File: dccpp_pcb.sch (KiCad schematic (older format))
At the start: 60 parts, among them J1 USB_B_Micro, J10 OSTTC022162, J11 OSTTC022162, J12 OSTTC022162, J2 AVR-ISP-6, J3 OSTTC022162, J4 OSTTC022162, J5 OSTTC022162, J6 OSTTC022162, J7 OSTTC022162, J8 OSTTC022162, J9 OSTTC022162, U1 ATmega32U4-AU, U2 74HC04, U3 IFX007T, U4 IFX007T, U5 IFX007T, U6 IFX007T, Y1 16MHz

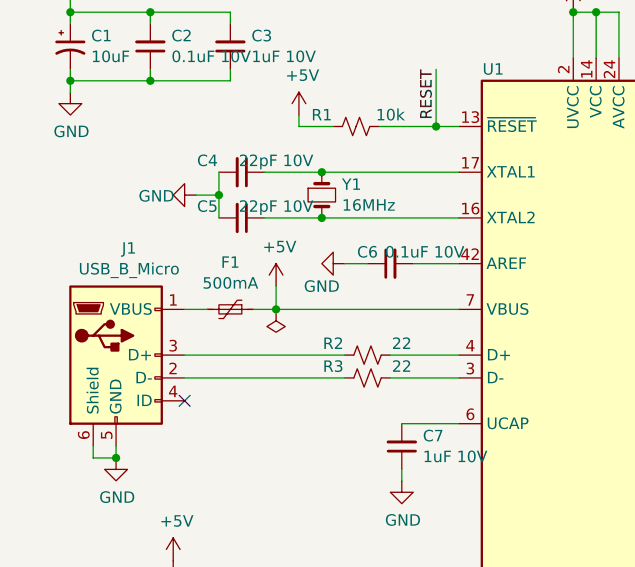
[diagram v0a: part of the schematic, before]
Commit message: Final part numbers
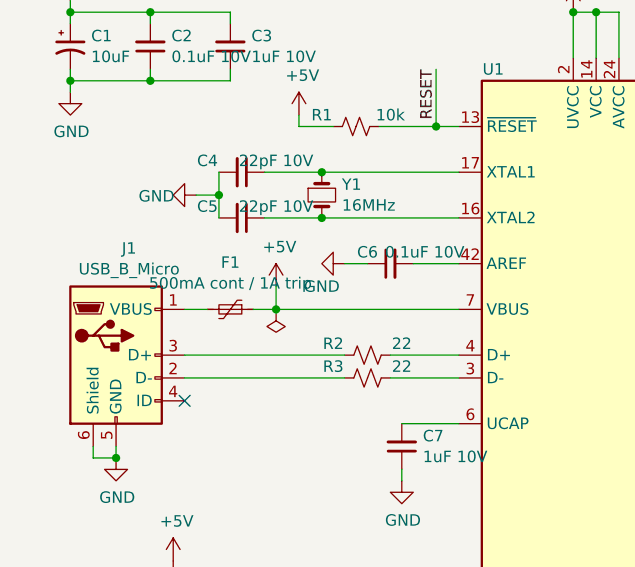
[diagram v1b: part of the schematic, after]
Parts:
- D1: Digi-Key_PN (none) -> 732-12018-1-ND; MPN (none) -> 150060YS55040
- D2: Digi-Key_PN (none) -> 732-12017-1-ND; MPN (none) -> 150060VS55040
- F1: value 500mA -> 500mA cont / 1A trip; footprint (none) -> Fuse:Fuse_1206_3216Metric_Pad1.42x1.75mm_HandSolder; Digi-Key_PN (none) -> 507-1802-1-ND; MPN (none) -> 0ZCJ0050FF2G
- J2: Digi-Key_PN (none) -> 609-5122-ND; MPN (none) -> 75869-331LF
- R1, R10, R11, R12, R13, R14, R15, R16, R6, R9: Digi-Key_PN (none) -> RNCP0603FTD10K0CT-ND; MPN (none) -> RNCP0603FTD10K0
- R17, R18, R19, R20: Digi-Key_PN (none) -> 311-510HRCT-ND; MPN (none) -> RC0603FR-07510RL
- R2, R3: Digi-Key_PN (none) -> 311-22.0HRCT-ND; MPN (none) -> RC0603FR-0722RL
- R4, R5: Digi-Key_PN (none) -> 311-330HRCT-ND; MPN (none) -> RC0603FR-07330RL
- R7, R8: Digi-Key_PN (none) -> 311-470HRCT-ND; MPN (none) -> RC0603FR-07470RL
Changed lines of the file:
@@
 F 2 "Resistor_SMD:R_0603_1608Metric_Pad1.05x0.95mm_HandSolder" H 2000 2400 50  0001 C CNN
 F 3 "~" H 2000 2400 50  0001 C CNN
+F 4 "311-22.0HRCT-ND" H 2000 2400 50  0001 C CNN "Digi-Key_PN"
+F 5 "RC0603FR-0722RL" H 2000 2400 50  0001 C CNN "MPN"
 	1    2000 2400
 	0    1    1    0
@@
 P 1400 2100
 F 0 "F1" V 1195 2100 50  0000 C CNN
-F 1 "500mA" V 1286 2100 50  0000 C CNN
-F 2 "" H 1450 1900 50  0001 L CNN
+F 1 "500mA cont / 1A trip" V 1286 2100 50  0000 C CNN
+F 2 "Fuse:Fuse_1206_3216Metric_Pad1.42x1.75mm_HandSolder" H 1450 1900 50  0001 L CNN
 F 3 "~" H 1400 2100 50  0001 C CNN
+F 4 "507-1802-1-ND" H 1400 2100 50  0001 C CNN "Digi-Key_PN"
+F 5 "0ZCJ0050FF2G" H 1400 2100 50  0001 C CNN "MPN"
 	1    1400 2100
 	0    1    1    0
@@
 F 2 "Resistor_SMD:R_0603_1608Metric_Pad1.05x0.95mm_HandSolder" H 1950 1300 50  0001 C CNN
 F 3 "~" H 1950 1300 50  0001 C CNN
+F 4 "RNCP0603FTD10K0CT-ND" H 1950 1300 50  0001 C CNN "Digi-Key_PN"
+F 5 "RNCP0603FTD10K0" H 1950 1300 50  0001 C CNN "MPN"
 	1    1950 1300
 	0    1    1    0
@@
 F 2 "Resistor_SMD:R_0603_1608Metric_Pad1.05x0.95mm_HandSolder" H 2000 2300 50  0001 C CNN
 F 3 "~" H 2000 2300 50  0001 C CNN
+F 4 "311-22.0HRCT-ND" H 2000 2300 50  0001 C CNN "Digi-Key_PN"
+F 5 "RC0603FR-0722RL" H 2000 2300 50  0001 C CNN "MPN"
 	1    2000 2300
 	0    1    1    0
@@
 F 2 "Connector_IDC:IDC-Header_2x03_P2.54mm_Vertical" V 1000 3750 50  0001 C CNN
 F 3 " ~" H -25 3150 50  0001 C CNN
+F 4 "609-5122-ND" H 1250 3700 50  0001 C CNN "Digi-Key_PN"
+F 5 "75869-331LF" H 1250 3700 50  0001 C CNN "MPN"
 	1    1250 3700
 	1    0    0    -1
@@
 F 2 "Resistor_SMD:R_0603_1608Metric_Pad1.05x0.95mm_HandSolder" H 9150 2100 50  0001 C CNN
 F 3 "~" H 9150 2100 50  0001 C CNN
+F 4 "311-510HRCT-ND" H 9150 2100 50  0001 C CNN "Digi-Key_PN"
+F 5 "RC0603FR-07510RL" H 9150 2100 50  0001 C CNN "MPN"
 	1    9150 2100
 	1    0    0    -1
@@
 F 2 "Resistor_SMD:R_0603_1608Metric_Pad1.05x0.95mm_HandSolder" H 9100 3000 50  0001 C CNN
 F 3 "~" H 9100 3000 50  0001 C CNN
+F 4 "311-510HRCT-ND" H 9100 3000 50  0001 C CNN "Digi-Key_PN"
+F 5 "RC0603FR-07510RL" H 9100 3000 50  0001 C CNN "MPN"
 	1    9100 3000
 	1    0    0    -1
@@
 F 2 "Resistor_SMD:R_0603_1608Metric_Pad1.05x0.95mm_HandSolder" H 9100 4100 50  0001 C CNN
 F 3 "~" H 9100 4100 50  0001 C CNN
+F 4 "311-510HRCT-ND" H 9100 4100 50  0001 C CNN "Digi-Key_PN"
+F 5 "RC0603FR-07510RL" H 9100 4100 50  0001 C CNN "MPN"
 	1    9100 4100
 	1    0    0    -1
@@
 F 2 "Resistor_SMD:R_0603_1608Metric_Pad1.05x0.95mm_HandSolder" H 9100 5000 50  0001 C CNN
 F 3 "~" H 9100 5000 50  0001 C CNN
+F 4 "311-510HRCT-ND" H 9100 5000 50  0001 C CNN "Digi-Key_PN"
+F 5 "RC0603FR-07510RL" H 9100 5000 50  0001 C CNN "MPN"
 	1    9100 5000
 	1    0    0    -1
@@
 F 2 "Resistor_SMD:R_0603_1608Metric_Pad1.05x0.95mm_HandSolder" H 9050 1700 50  0001 C CNN
 F 3 "~" H 9050 1700 50  0001 C CNN
+F 4 "RNCP0603FTD10K0CT-ND" H 9050 1700 50  0001 C CNN "Digi-Key_PN"
+F 5 "RNCP0603FTD10K0" H 9050 1700 50  0001 C CNN "MPN"
 	1    9050 1700
 	0    1    1    0
@@
 F 2 "Resistor_SMD:R_0603_1608Metric_Pad1.05x0.95mm_HandSolder" H 9050 1800 50  0001 C CNN
 F 3 "~" H 9050 1800 50  0001 C CNN
+F 4 "RNCP0603FTD10K0CT-ND" H 9050 1800 50  0001 C CNN "Digi-Key_PN"
+F 5 "RNCP0603FTD10K0" H 9050 1800 50  0001 C CNN "MPN"
 	1    9050 1800
 	0    1    1    0
@@
 F 2 "Resistor_SMD:R_0603_1608Metric_Pad1.05x0.95mm_HandSolder" H 9050 2600 50  0001 C CNN
 F 3 "~" H 9050 2600 50  0001 C CNN
+F 4 "RNCP0603FTD10K0CT-ND" H 9050 2600 50  0001 C CNN "Digi-Key_PN"
+F 5 "RNCP0603FTD10K0" H 9050 2600 50  0001 C CNN "MPN"
 	1    9050 2600
 	0    1    1    0
@@
 F 2 "Resistor_SMD:R_0603_1608Metric_Pad1.05x0.95mm_HandSolder" H 9050 2700 50  0001 C CNN
 F 3 "~" H 9050 2700 50  0001 C CNN
+F 4 "RNCP0603FTD10K0CT-ND" H 9050 2700 50  0001 C CNN "Digi-Key_PN"
+F 5 "RNCP0603FTD10K0" H 9050 2700 50  0001 C CNN "MPN"
 	1    9050 2700
 	0    1    1    0
@@
 F 2 "Resistor_SMD:R_0603_1608Metric_Pad1.05x0.95mm_HandSolder" H 9050 3700 50  0001 C CNN
 F 3 "~" H 9050 3700 50  0001 C CNN
+F 4 "RNCP0603FTD10K0CT-ND" H 9050 3700 50  0001 C CNN "Digi-Key_PN"
+F 5 "RNCP0603FTD10K0" H 9050 3700 50  0001 C CNN "MPN"
 	1    9050 3700
 	0    1    1    0
@@
 F 2 "Resistor_SMD:R_0603_1608Metric_Pad1.05x0.95mm_HandSolder" H 9050 3800 50  0001 C CNN
 F 3 "~" H 9050 3800 50  0001 C CNN
+F 4 "RNCP0603FTD10K0CT-ND" H 9050 3800 50  0001 C CNN "Digi-Key_PN"
+F 5 "RNCP0603FTD10K0" H 9050 3800 50  0001 C CNN "MPN"
 	1    9050 3800
 	0    1    1    0
@@
 F 2 "Resistor_SMD:R_0603_1608Metric_Pad1.05x0.95mm_HandSolder" H 9050 4600 50  0001 C CNN
 F 3 "~" H 9050 4600 50  0001 C CNN
+F 4 "RNCP0603FTD10K0CT-ND" H 9050 4600 50  0001 C CNN "Digi-Key_PN"
+F 5 "RNCP0603FTD10K0" H 9050 4600 50  0001 C CNN "MPN"
 	1    9050 4600
 	0    1    1    0
@@
 F 2 "Resistor_SMD:R_0603_1608Metric_Pad1.05x0.95mm_HandSolder" H 9050 4700 50  0001 C CNN
 F 3 "~" H 9050 4700 50  0001 C CNN
+F 4 "RNCP0603FTD10K0CT-ND" H 9050 4700 50  0001 C CNN "Digi-Key_PN"
+F 5 "RNCP0603FTD10K0" H 9050 4700 50  0001 C CNN "MPN"
 	1    9050 4700
 	0    1    1    0
@@
 F 2 "LED_SMD:LED_0603_1608Metric_Pad1.05x0.95mm_HandSolder" H 4300 3000 50  0001 C CNN
 F 3 "~" H 4300 3000 50  0001 C CNN
+F 4 "732-12017-1-ND" H 4300 3000 50  0001 C CNN "Digi-Key_PN"
+F 5 "150060VS55040" H 4300 3000 50  0001 C CNN "MPN"
 	1    4300 3000
 	1    0    0    -1
@@
 F 2 "Resistor_SMD:R_0603_1608Metric_Pad1.05x0.95mm_HandSolder" H 3800 3000 50  0001 C CNN
 F 3 "~" H 3800 3000 50  0001 C CNN
+F 4 "311-330HRCT-ND" H 3800 3000 50  0001 C CNN "Digi-Key_PN"
+F 5 "RC0603FR-07330RL" H 3800 3000 50  0001 C CNN "MPN"
 	1    3800 3000
 	0    1    1    0
@@
 F 2 "Resistor_SMD:R_0603_1608Metric_Pad1.05x0.95mm_HandSolder" H 3800 1300 50  0001 C CNN
 F 3 "~" H 3800 1300 50  0001 C CNN
+F 4 "311-330HRCT-ND" H 3800 1300 50  0001 C CNN "Digi-Key_PN"
+F 5 "RC0603FR-07330RL" H 3800 1300 50  0001 C CNN "MPN"
 	1    3800 1300
 	0    1    1    0
@@
 F 2 "LED_SMD:LED_0603_1608Metric_Pad1.05x0.95mm_HandSolder" H 4300 1300 50  0001 C CNN
 F 3 "~" H 4300 1300 50  0001 C CNN
+F 4 "732-12018-1-ND" H 4300 1300 50  0001 C CNN "Digi-Key_PN"
+F 5 "150060YS55040" H 4300 1300 50  0001 C CNN "MPN"
 	1    4300 1300
 	1    0    0    -1
@@
 F 2 "Resistor_SMD:R_0603_1608Metric_Pad1.05x0.95mm_HandSolder" H 8300 4900 50  0001 C CNN
 F 3 "~" H 8300 4900 50  0001 C CNN
+F 4 "311-470HRCT-ND" H 8300 4900 50  0001 C CNN "Digi-Key_PN"
+F 5 "RC0603FR-07470RL" H 8300 4900 50  0001 C CNN "MPN"
 	1    8300 4900
 	1    0    0    -1
@@
 F 2 "Resistor_SMD:R_0603_1608Metric_Pad1.05x0.95mm_HandSolder" H 8300 2900 50  0001 C CNN
 F 3 "~" H 8300 2900 50  0001 C CNN
+F 4 "311-470HRCT-ND" H 8300 2900 50  0001 C CNN "Digi-Key_PN"
+F 5 "RC0603FR-07470RL" H 8300 2900 50  0001 C CNN "MPN"
 	1    8300 2900
 	1    0    0    -1
@@
 F 2 "Resistor_SMD:R_0603_1608Metric_Pad1.05x0.95mm_HandSolder" H 4400 3400 50  0001 C CNN
 F 3 "~" H 4400 3400 50  0001 C CNN
+F 4 "RNCP0603FTD10K0CT-ND" H 4400 3400 50  0001 C CNN "Digi-Key_PN"
+F 5 "RNCP0603FTD10K0" H 4400 3400 50  0001 C CNN "MPN"
 	1    4400 3400
 	0    1    1    0
